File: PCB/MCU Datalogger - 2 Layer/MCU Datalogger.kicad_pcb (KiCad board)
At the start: 2 copper layers, 50.8 x 30.5 mm, 29 parts, among them J1 Conn_01x04_Pin, J2 Conn_01x04_Pin, J3 Conn_01x09_Pin, J4 Conn_02x03_Odd_Even, U1 24LC1025, U2 24LC1025, U3 DS1337S+, U4 ATMEGA328P-AU, Y1 16 MHz, Y2 32.768 Khz

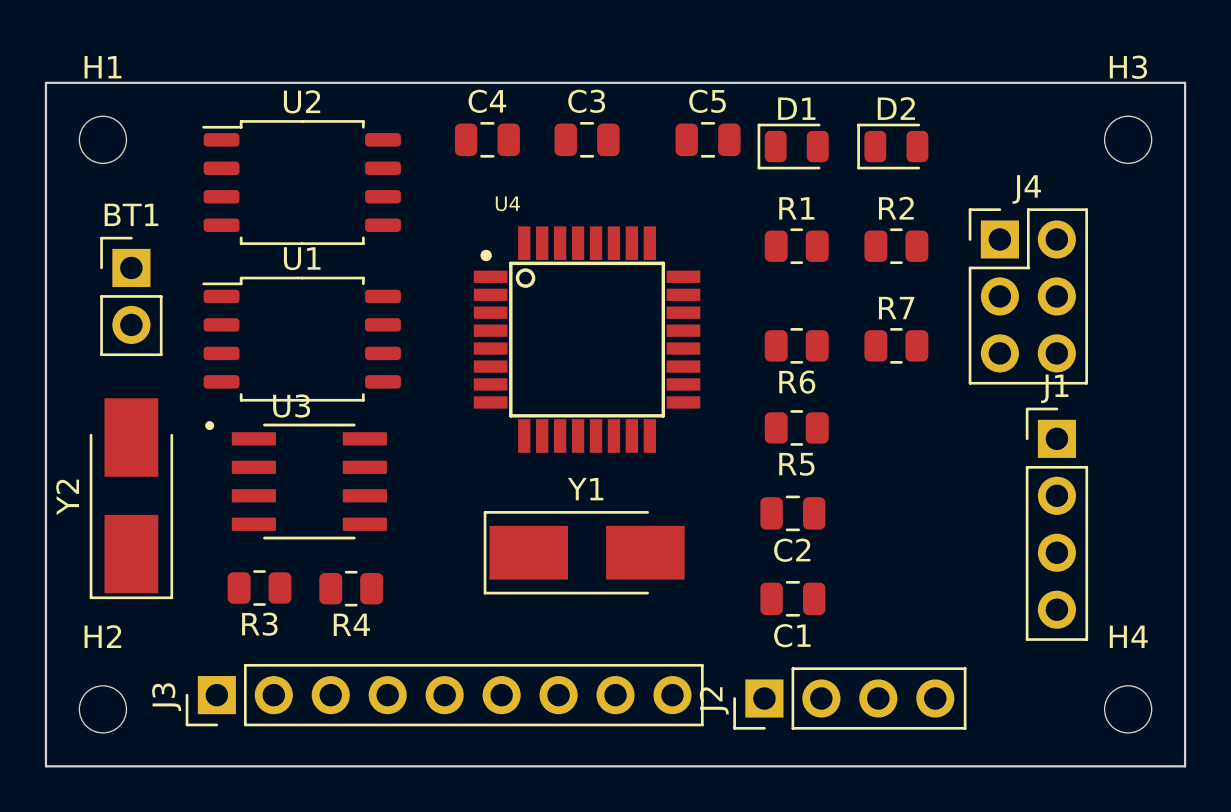
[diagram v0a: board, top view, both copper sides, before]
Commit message: Route
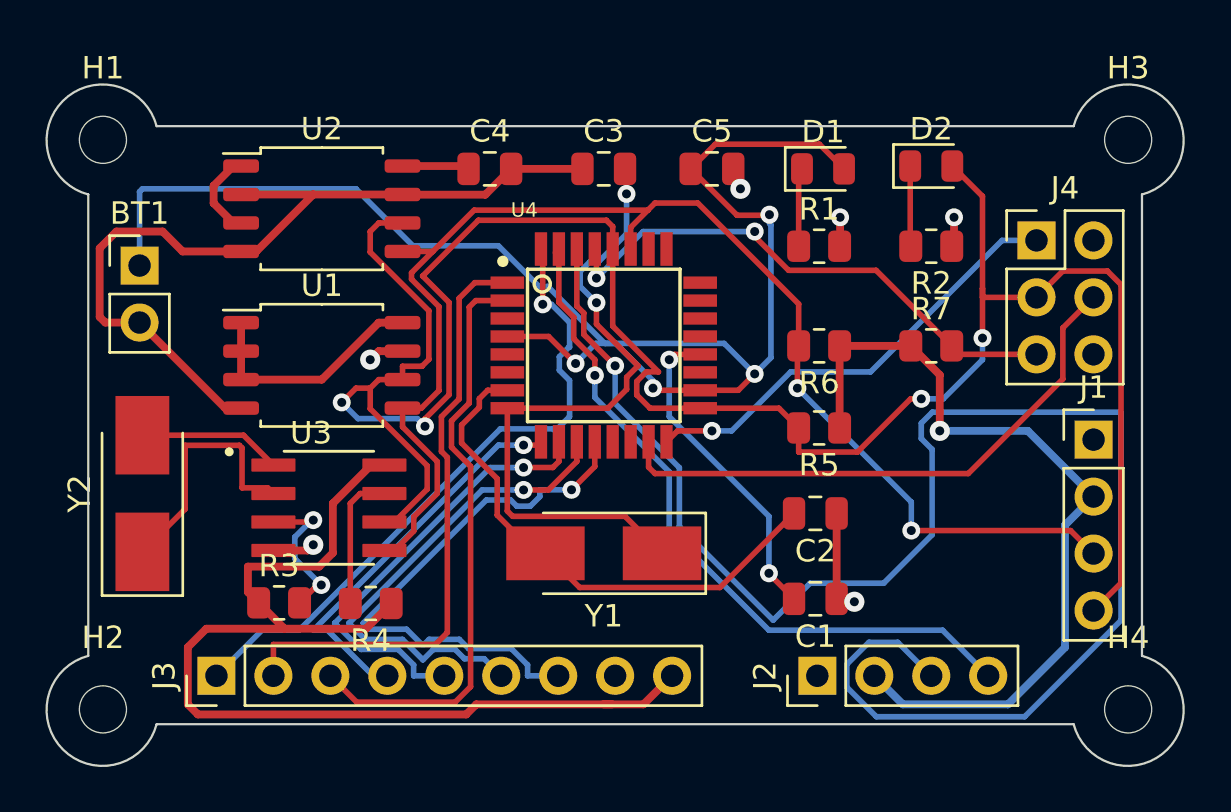
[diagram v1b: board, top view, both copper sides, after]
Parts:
- moved J2 2.57 mm to (157.7, 114.4)
- moved D2 1.78 mm to (162.8, 91.7)
- moved J4 1.63 mm to (167.5, 95.0)
- moved J1 1.63 mm to (170.1, 103.9)
- moved R2 1.55 mm to (162.8, 95.3), turned to 180 degrees
- moved R7 1.55 mm to (162.8, 99.7)
- moved D1 1.54 mm to (158.0, 91.8)
- moved C3 1.49 mm to (148.2, 91.8)
- moved U1 1.46 mm to (135.6, 100.6)
- moved U2 1.46 mm to (135.6, 93.6)
- moved U3 1.46 mm to (136.0, 106.9)
- moved C5 1.31 mm to (153.0, 91.8)
- moved C4 1.30 mm to (143.1, 91.8)
- moved R4 1.09 mm to (137.8, 111.2)
- moved R3 1.09 mm to (133.7, 111.2), turned to 0 degrees
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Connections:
- R5 pad 1: Net-(R5-Pad1) -> /Vcc
- R6 pad 1: Net-(R5-Pad1) -> /Vcc
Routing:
- net /Vcc: track 0.00 -> 102.5 mm, vias 0 -> 1
- net /SCK: track 0.00 -> 102.3 mm, vias 0 -> 4
- net /RX: track 0.00 -> 72.8 mm, vias 0 -> 1
- net Net-(BT1-+): track 0.00 -> 67.0 mm, vias 0 -> 4
- net /SDA: track 0.00 -> 60.5 mm, vias 0 -> 2
- net GND: track 0.00 -> 50.1 mm, vias 0 -> 6
- net /TX: track 0.00 -> 32.0 mm, vias 0 -> 1
- net Net-(U4-PB7): track 0.00 -> 30.5 mm, vias 0 -> 2
- net /D2: track 0.00 -> 29.2 mm, vias 0 -> 1
- net /D3: track 0.00 -> 27.2 mm
- net /D4: track 0.00 -> 26.5 mm
- net /MOSI: track 0.00 -> 25.7 mm
- net /D8: track 0.00 -> 24.9 mm, vias 0 -> 1
- net /RESET: track 0.00 -> 24.2 mm, vias 0 -> 2
- net Net-(U4-PB6): track 0.00 -> 23.5 mm
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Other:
- board size 50.8 x 30.5 mm -> 50.7 x 30.4 mm
